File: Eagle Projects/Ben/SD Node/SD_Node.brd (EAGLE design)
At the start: 93 x 90 mm, 33 parts, among them Q1 16MHz, Q3 16MHz, Q4 16MHz, Q5 16MHz, U1 ATMEGA328P_TQFP, U2 MCP2551, X1 5566-6, X2 5566-6

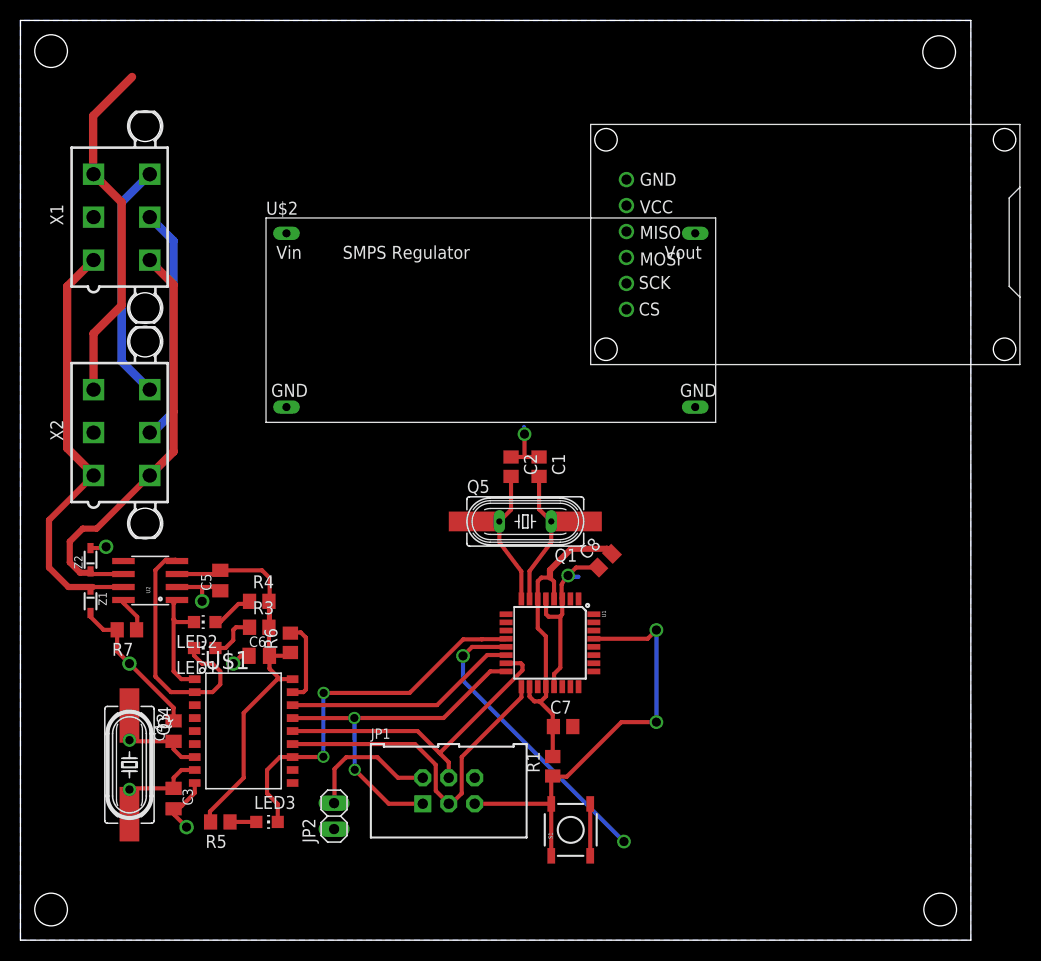
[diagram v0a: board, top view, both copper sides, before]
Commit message: SD Node Done?
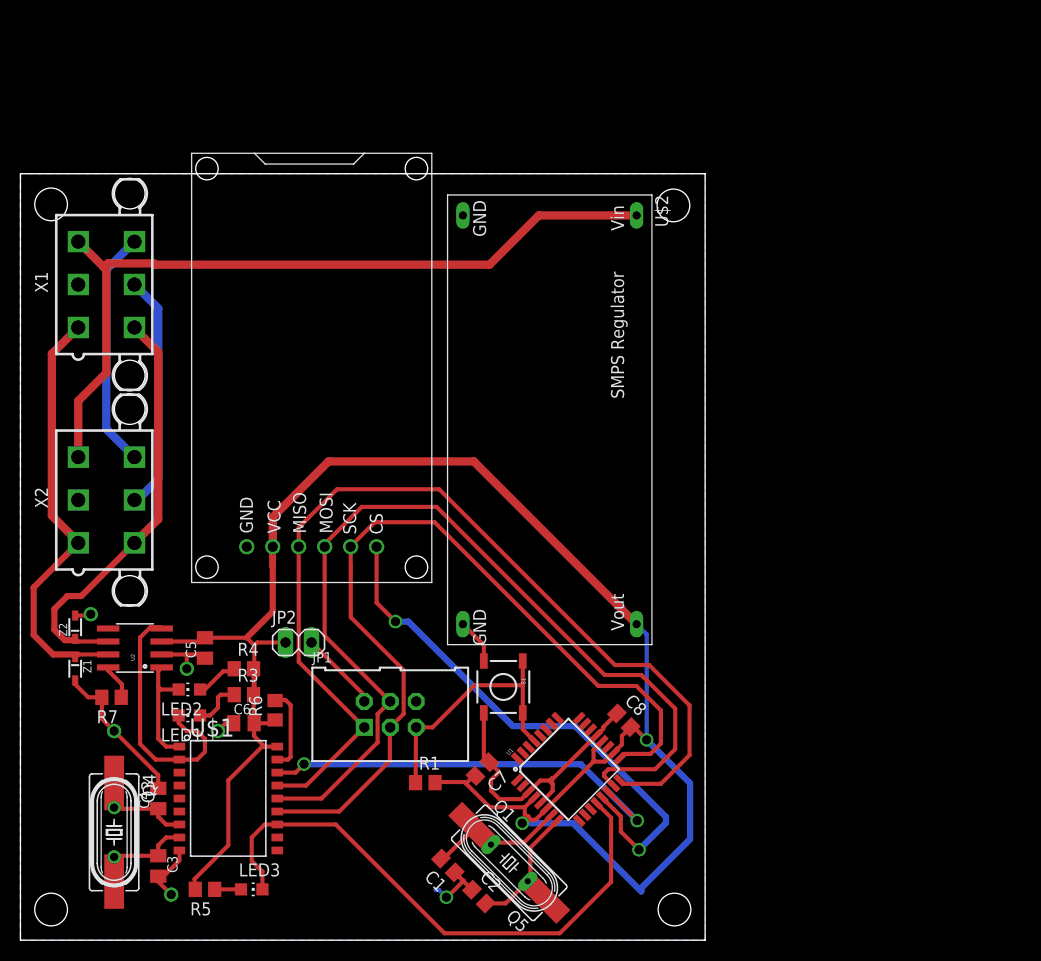
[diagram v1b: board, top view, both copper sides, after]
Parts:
- moved C2 42.2 mm to (44.9, 4.27), turned to 315 degrees
- moved C1 40.0 mm to (41.8, 7.31), turned to 135 degrees
- moved Q1 33.5 mm to (47.8, 7.56), turned to 315 degrees
- moved Q5 33.4 mm to (47.8, 7.57), turned to 135 degrees
- moved U$2 28.5 mm to (41.8, 72.9), turned to 270 degrees
- moved U$3 26.4 mm to (40.2, 35.0), turned to 90 degrees
- moved JP2 17.3 mm to (27.2, 29.1), turned to 0 degrees
- moved C8 15.7 mm to (59.0, 21.5), turned to 315 degrees
- moved S1 15.5 mm to (47.3, 24.8), turned to 270 degrees
- moved R1 12.6 mm to (39.6, 15.4), turned to 0 degrees
- moved U1 12.5 mm to (53.6, 16.7), turned to 45 degrees
- moved JP1 9.42 mm to (36.2, 22.1)
- moved C7 8.92 mm to (45.2, 16.8), turned to 225 degrees
- moved X1 6.77 mm to (8.41, 64.2)
- moved C5 6.77 mm to (18.1, 28.6)
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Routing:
- net +5V: track 76.4 -> 186.9 mm, vias 0 -> 2
- net MOSI: track 31.7 -> 92.2 mm
- net MISO: track 35.9 -> 94.7 mm, vias 2 -> 0
- net SCK: track 33.8 -> 83.6 mm
- net +12V: track 34.5 -> 77.8 mm
- net SD_CS: track 29.3 -> 53.4 mm
- net CANCS: track 22.9 -> 41.9 mm, vias 0 -> 2
- net CANINT: track 37.9 -> 56.0 mm, vias 2 -> 0
- net RST: track 43.2 -> 25.9 mm, vias 2 -> 0
- net GND: track 59.2 -> 69.1 mm, vias 7 -> 6
- net N$10: track 13.3 -> 7.90 mm
- net N$1: track 15.7 -> 14.0 mm
- net N$2: track 15.5 -> 14.8 mm
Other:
- board size 93 x 90 mm -> 67 x 75 mm
